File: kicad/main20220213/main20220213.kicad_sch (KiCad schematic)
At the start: 64 parts, among them J1 MD2, J10 micro-b_in, J11 I2C_ToF, J12 I2C_OLED, J13 drib-kick, J14 Power IN, J15 LINE, J16 MD1, J17 MD2, J18 MD3, J19 MD4, J2 MD4, J20 Drib-Kick, J21 Trimmer, J3 MD3, J4 MD1, J5 XBee, J6 Serial3/Vision, J7 raspi-power, J8 Serial2/IMU, J9 micro-b_out, Q1 AO3400A, Q2 AO3401A, SW1 PROG, SW2 Reset, SW3 SET, SW4 SW_SPST, U1 OKL-T_3-W12N-C, U2 Teensy3.5, U3 74HC32, U4 74HC04

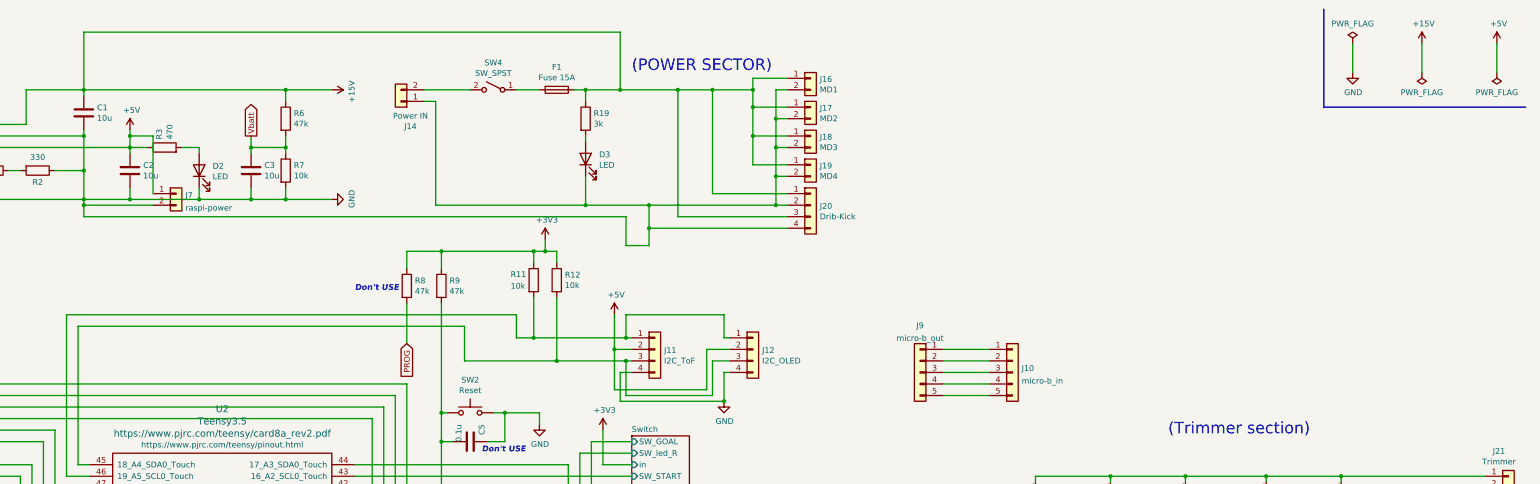
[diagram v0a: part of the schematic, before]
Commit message: pcb
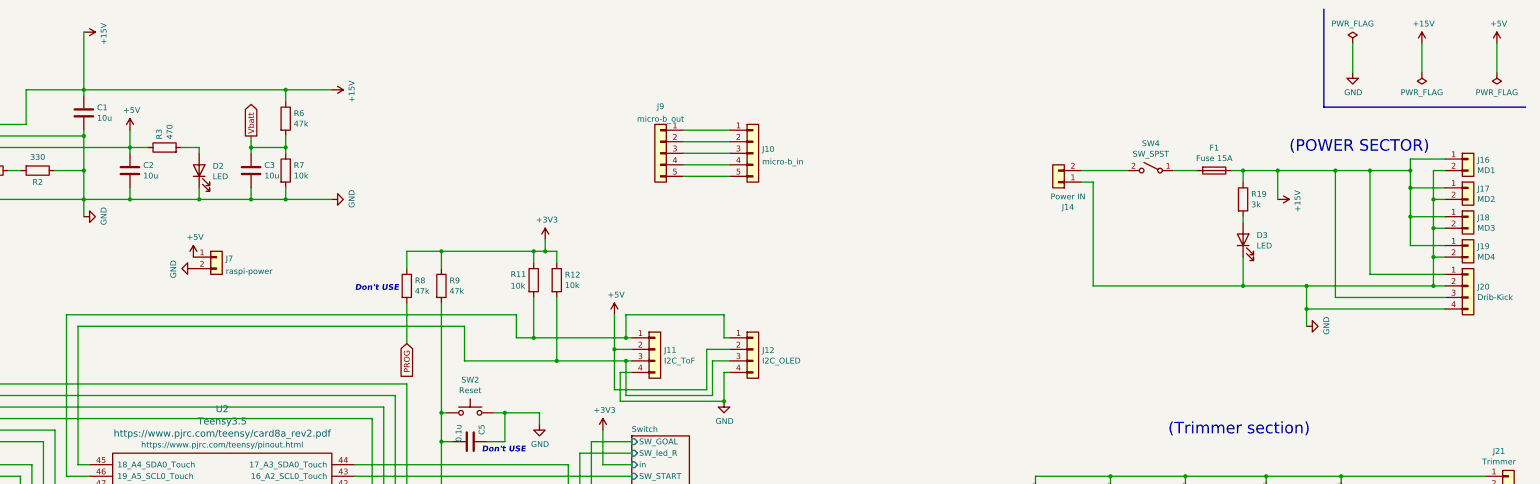
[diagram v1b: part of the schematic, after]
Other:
- moved on the sheet: D3, F1, J10, J14, J16, J17, J18, J19, J20, J7, J9, R19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
